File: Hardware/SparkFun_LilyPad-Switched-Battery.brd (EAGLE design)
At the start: 29.4 x 29.2 mm, 12 parts

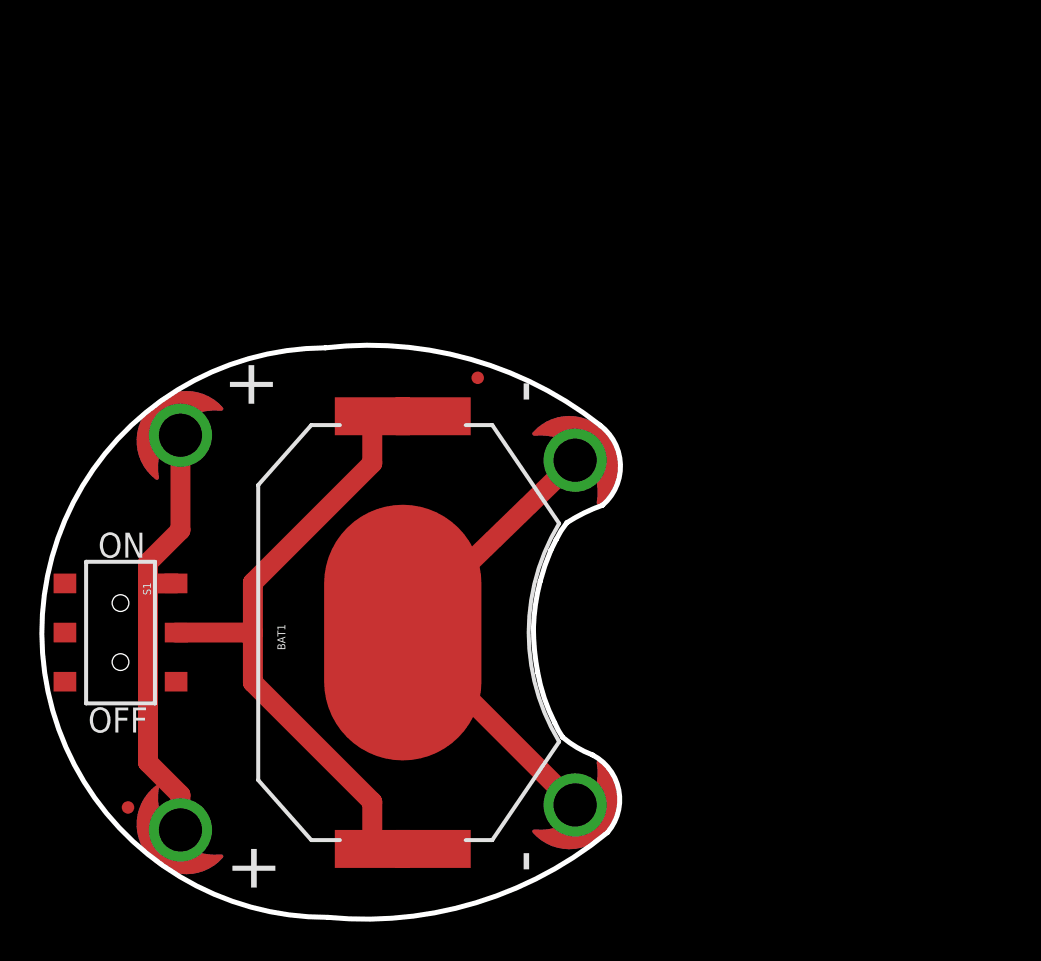
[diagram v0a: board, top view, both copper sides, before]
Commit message: Updated Board and Schematic files
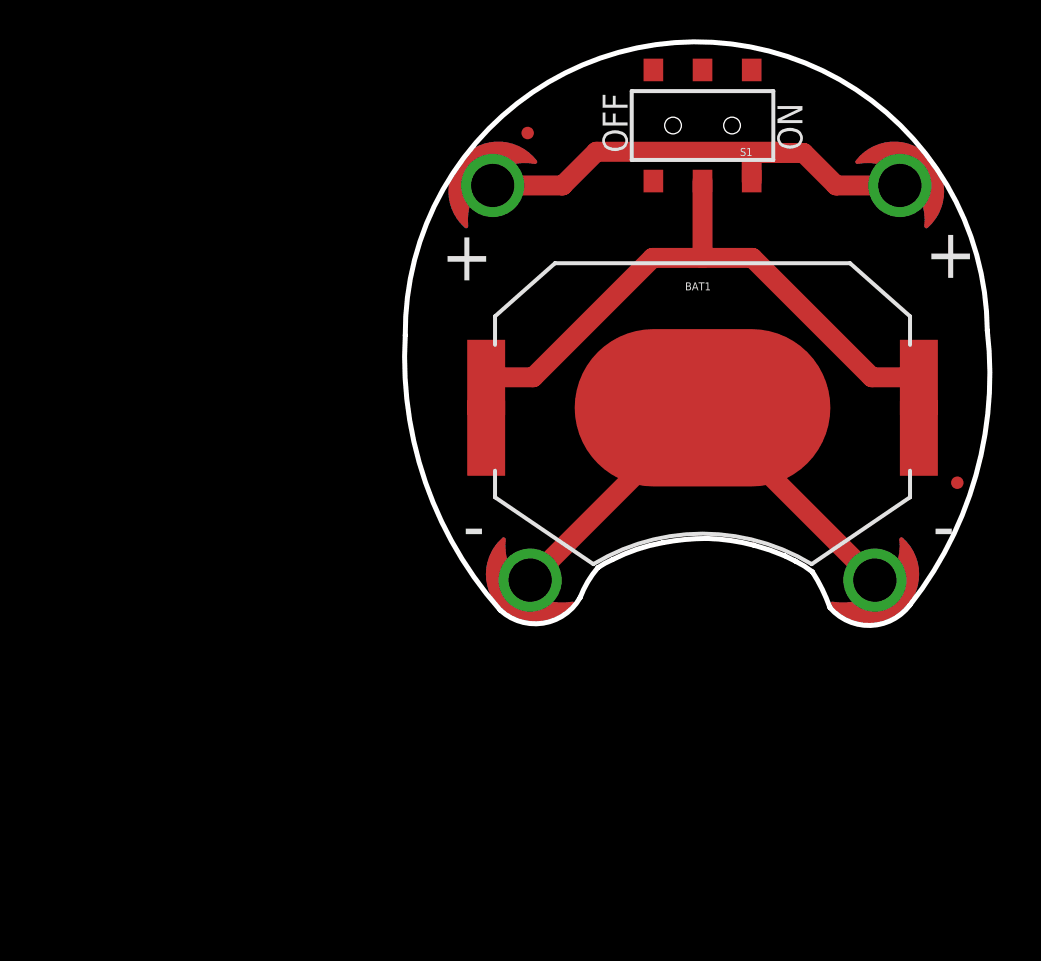
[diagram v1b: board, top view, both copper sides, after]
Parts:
- added U$1: REVISION, SparkFun-Aesthetics:REVISION
- moved FRAME1 92.0 mm to (-21.8, -10.2)
- moved U$7 42.3 mm to (20.6, 25.8), turned to 0 degrees
- moved JP1 39.9 mm to (6.35, 25.4), turned to 270 degrees
- moved S1 39.2 mm to (15.2, 25.8), turned to 180 degrees
- moved ST4 38.7 mm to (25.3, 22.7), turned to 137 degrees
- moved ST3 36.4 mm to (4.57, 22.7), turned to 223 degrees
- moved LOGO1 34.9 mm to (11.4, 24.2), turned to 0 degrees
- moved JP2 25.0 mm to (28.2, 7.62), turned to 270 degrees
- moved U$5 24.4 mm to (15.2, 15.2), turned to 0 degrees
- moved BAT1 19.1 mm to (15.2, 11.4), turned to 0 degrees
- moved ST2 16.4 mm to (24.0, 2.67), turned to 43 degrees
- moved ST1 11.7 mm to (6.48, 2.67), turned to 317 degrees
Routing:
- net N$1: track 22.9 -> 24.8 mm
- net N$2: track 26.1 -> 24.9 mm
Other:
- board size 29.4 x 29.2 mm -> 29.8 x 29.7 mm
- board text added: "Jim Lindblom"
- board text added: "Mary West"
